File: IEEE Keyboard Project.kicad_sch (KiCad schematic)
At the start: 122 parts, among them U1 RP2354B

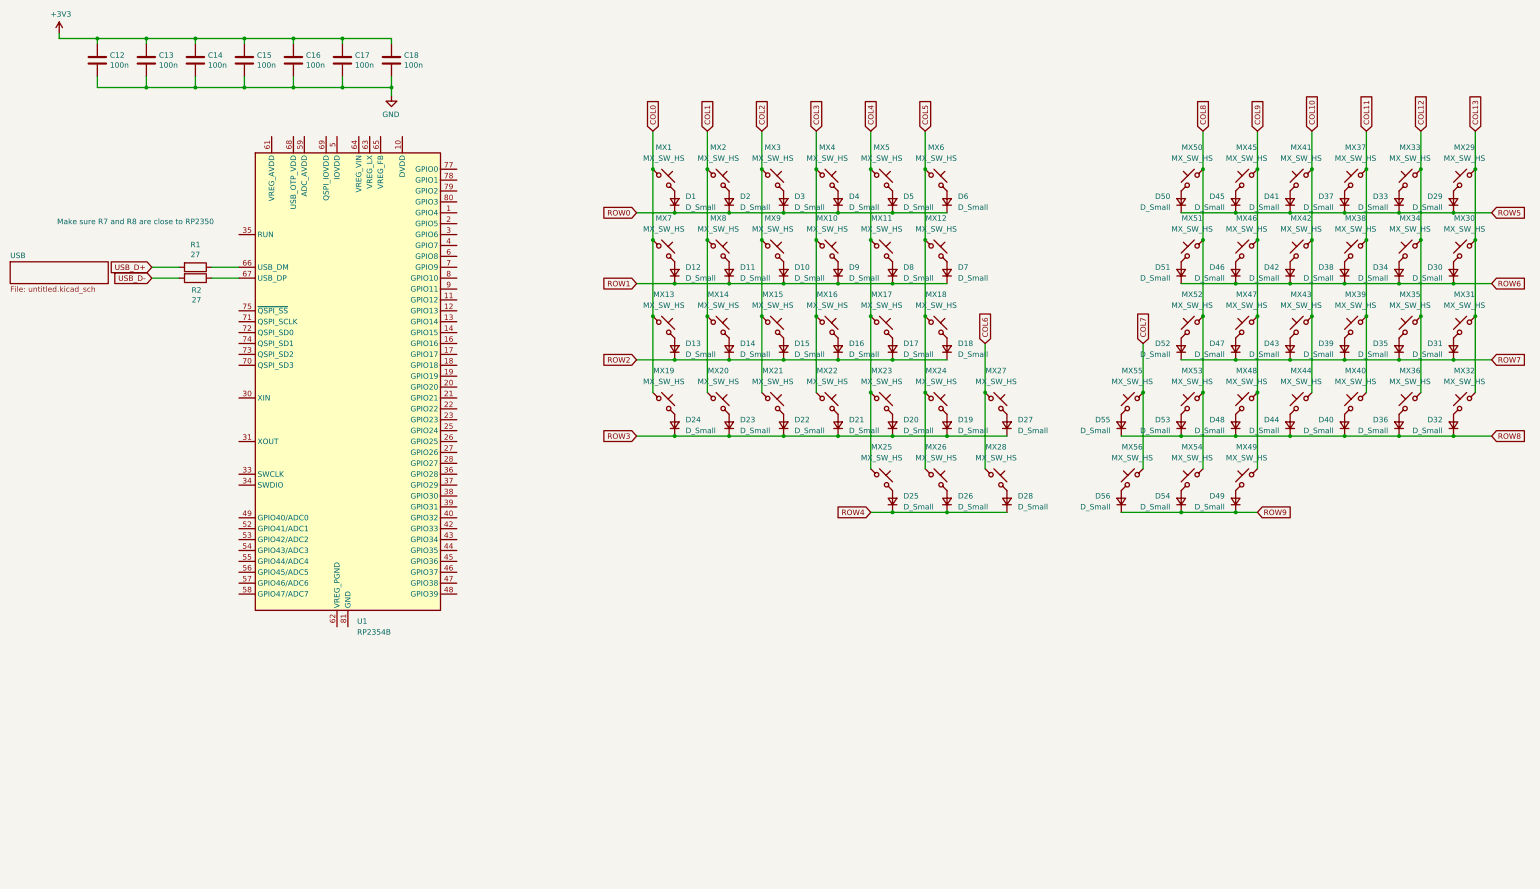
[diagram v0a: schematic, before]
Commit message: Add files via upload
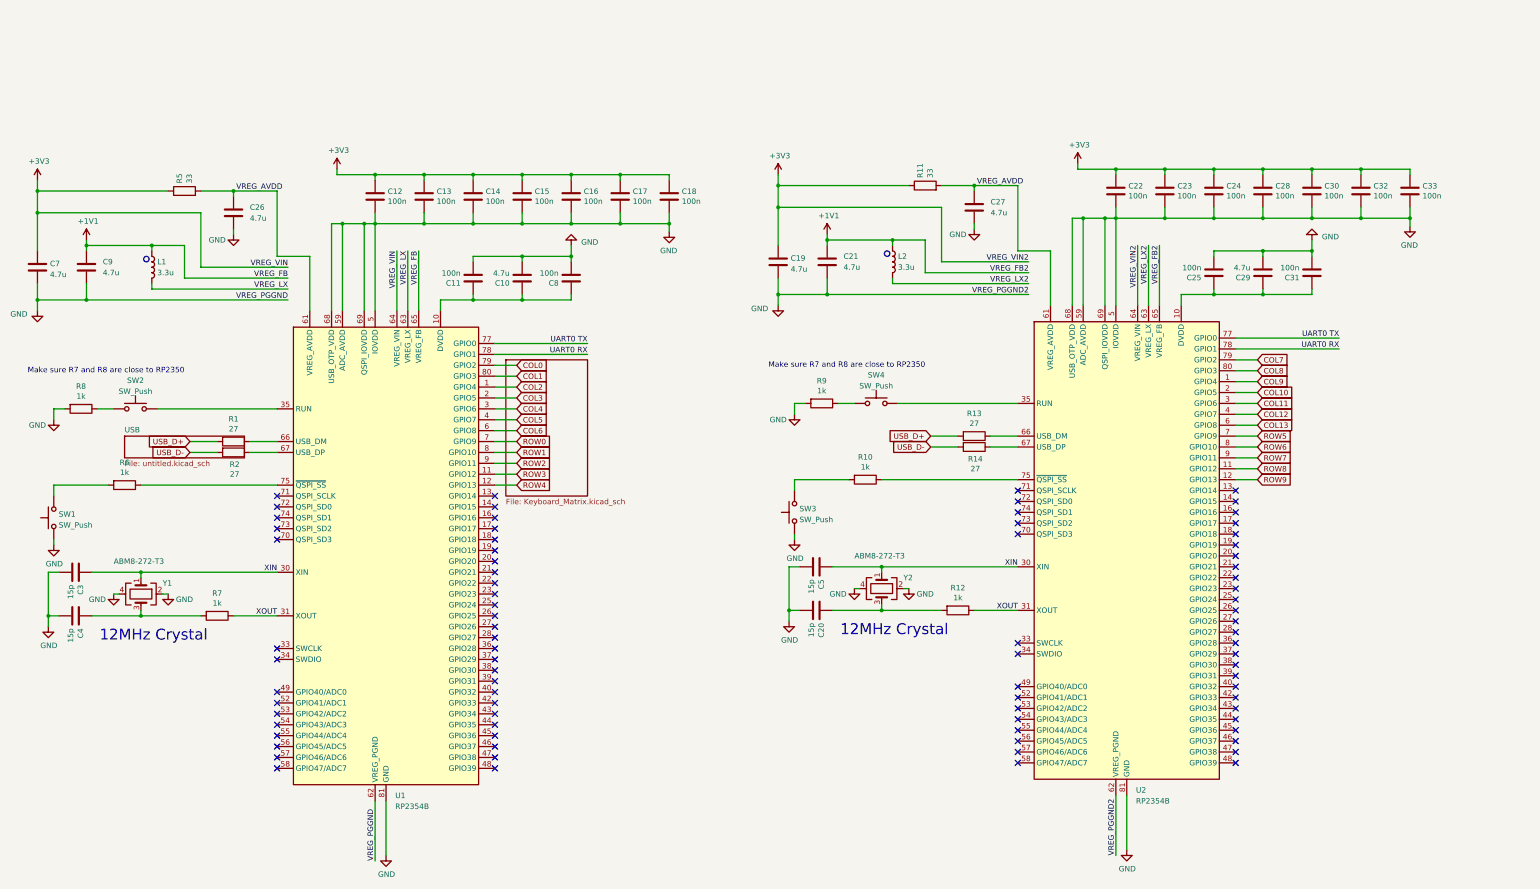
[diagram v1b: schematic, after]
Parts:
- removed D1, D10, D11, D12, D13, D14, D15, D16, D17, D18, D19, D2, D20, D21, D22, D23, D24, D25, D26, D27, D28, D29, D3, D30, D31, D32, D33, D34, D35, D36, D37, D38, D39, D4, D40, D41, D42, D43, D44, D45, D46, D47, D48, D49, D5, D50, D51, D52, D53, D54, D55, D56, D6, D7, D8, D9: D_Small, symbol Device:D_Small
- removed MX1, MX10, MX11, MX12, MX13, MX14, MX15, MX16, MX17, MX18, MX19, MX2, MX20, MX21, MX22, MX23, MX24, MX25, MX26, MX27, MX28, MX29, MX3, MX30, MX31, MX32, MX33, MX34, MX35, MX36, MX37, MX38, MX39, MX4, MX40, MX41, MX42, MX43, MX44, MX45, MX46, MX47, MX48, MX49, MX5, MX50, MX51, MX52, MX53, MX54, MX55, MX56, MX6, MX7, MX8, MX9: MX_SW_HS, Button_Switch_Keyboard:SW_Cherry_MX_1.00u_PCB, symbol marbastlib-mx:MX_SW_HS_CPG151101S11
- added C10, C26, C27, C29: 4.7u, Capacitor_SMD:C_0402_1005Metric, symbol Device:C
- added C11, C22, C23, C24, C25, C28, C30, C31, C32, C33, C8: 100n, Capacitor_SMD:C_0402_1005Metric, symbol Device:C
- added C19, C21, C7, C9: 4.7u, RP2350_60QFN_minimal:C_0402_1005Metric_small_pads, symbol Device:C
- added C20, C3, C4, C5: 15p, Capacitor_SMD:C_0402_1005Metric, symbol Device:C
- added L1, L2: 3.3u, RP2350_60QFN_minimal:L_pol_2016, symbol Device:L
- added R10, R12, R6, R7, R8, R9: 1k, Resistor_SMD:R_0402_1005Metric, symbol Device:R
- added R11, R5: 33, Resistor_SMD:R_0402_1005Metric, symbol Device:R
- added R13, R14: 27, Resistor_SMD:R_0402_1005Metric, symbol Device:R
- added SW1, SW2, SW3, SW4: SW_Push, Button_Switch_SMD:SW_Push_1P1T_NO_Vertical_Wuerth_434133025816, symbol Switch:SW_Push
- added U2: RP2354B, Package_DFN_QFN:QFN-80-1EP_10x10mm_P0.4mm_EP3.4x3.4mm, symbol MCU_RaspberryPi:RP2354B
- added Y1, Y2: ABM8-272-T3, Crystal:Crystal_SMD_3225-4Pin_3.2x2.5mm, symbol Device:Crystal_GND24
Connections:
- net +3V3: now also U1.64 (VREG_VIN), C19.1, C22.1, C23.1, C24.1, C28.1, C30.1, C32.1, C33.1, C7.1, R11.1, R5.1, U2.64 (VREG_VIN)
- net COL0: now also U1.79 (GPIO2)
- net COL1: now also U1.80 (GPIO3)
- net COL10: now also U2.2 (GPIO5)
- net COL11: now also U2.3 (GPIO6)
- net COL12: now also U2.4 (GPIO7)
- net COL13: now also U2.6 (GPIO8)
- net COL2: now also U1.1 (GPIO4)
- net COL3: now also U1.2 (GPIO5)
- net COL4: now also U1.3 (GPIO6)
- net COL5: now also U1.4 (GPIO7)
- net COL6: now also U1.6 (GPIO8)
- net COL7: now also U2.79 (GPIO2)
- net COL8: now also U2.80 (GPIO3)
- net COL9: now also U2.1 (GPIO4)
- net GND: now also U1.15 (IOVDD), U1.24 (IOVDD), U1.29 (IOVDD), U1.41 (IOVDD), U1.5 (IOVDD), U1.50 (IOVDD), U1.59 (ADC_AVDD), U1.60 (IOVDD), U1.62 (VREG_PGND), U1.68 (USB_OTP_VDD), U1.69 (QSPI_IOVDD), U1.76 (IOVDD), U1.81 (GND), C10.2, C11.2, C19.2, C20.2, C21.2, C22.2, C23.2, C24.2, C25.2, C26.2, C27.2, C28.2, C29.2, C3.2, C30.2, C31.2, C32.2, C33.2, C4.2, C5.2, C7.2, C8.2, C9.2, R8.2, R9.2, SW1.1, SW3.1, U2.15 (IOVDD), U2.24 (IOVDD), U2.29 (IOVDD), U2.41 (IOVDD), U2.5 (IOVDD), U2.50 (IOVDD), U2.59 (ADC_AVDD), U2.60 (IOVDD), U2.62 (VREG_PGND), U2.68 (USB_OTP_VDD), U2.69 (QSPI_IOVDD), U2.76 (IOVDD), U2.81 (GND), Y1.2, Y1.4, Y2.2, Y2.4
- net ROW0: now also U1.7 (GPIO9)
- net ROW1: now also U1.8 (GPIO10)
- net ROW2: now also U1.9 (GPIO11)
- net ROW3: now also U1.11 (GPIO12)
- net ROW4: now also U1.12 (GPIO13)
- net ROW5: now also U2.7 (GPIO9)
- net ROW6: now also U2.8 (GPIO10)
- net ROW7: now also U2.9 (GPIO11)
- net ROW8: now also U2.11 (GPIO12)
- net ROW9: now also U2.12 (GPIO13)
- net USB_D+: now also R13.2
- net USB_D-: now also R14.2
- net at U1.10 (DVDD), U1.32 (DVDD), U1.51 (DVDD): now also C10.1, C11.1, C8.1
- net XIN: now reaches U1.30 (XIN)
- net XIN: now also C3.1, C5.1, U2.30 (XIN), Y1.1, Y2.1
- net XOUT: now reaches U1.31 (XOUT)
- net XOUT: now also R12.1, R7.1, U2.31 (XOUT)
- net at U1.35 (RUN): now also SW2.2
- net VREG_AVDD: now reaches U1.61 (VREG_AVDD)
- net VREG_AVDD: now also C26.1, C27.1, R11.2, R5.2, U2.61 (VREG_AVDD)
- net VREG_LX: now reaches U1.63 (VREG_LX)
- net VREG_LX: now also L1.2
- net +1V1: now reaches U1.65 (VREG_FB)
- net +1V1: now also C21.1, C9.1, L1.1, L2.1, U2.65 (VREG_FB)
- net at U1.75 (~{QSPI_SS}): now also R6.1
- net UART0 TX: now reaches U1.77 (GPIO0)
- net UART0 TX: now also U2.77 (GPIO0)
- net UART0 RX: now reaches U1.78 (GPIO1)
- net UART0 RX: now also U2.78 (GPIO1)
- new net: C25.1, C29.1, C31.1, U2.10 (DVDD), U2.32 (DVDD), U2.51 (DVDD)
- new net: R9.1, SW4.1
- new net: SW4.2, U2.35 (RUN)
- new net: R10.1, U2.75 (~{QSPI_SS})
- new net: R10.2, SW3.2
- new net: R8.1, SW2.1
- new net: C20.1, R12.2, Y2.3
- new net: R6.2, SW1.2
- new net: C4.1, R7.2, Y1.3
- new net: R13.1, U2.66 (USB_DM)
- new net: R14.1, U2.67 (USB_DP)
- new net VREG_LX2: L2.2, U2.63 (VREG_LX)
- no-connect marks 0 -> 82
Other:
- added sheet Keyboard Matrix (Keyboard_Matrix.kicad_sch)
- note added: "12MHz Crystal"
- moved on the sheet: C12, C13, C14, C15, C16, C17, C18, R1, R2, U1
